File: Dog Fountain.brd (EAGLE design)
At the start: 88.6 x 53.3 mm, 19 parts, among them IC1 L298, J1 22-27-2021-02, J4 22-27-2021-02

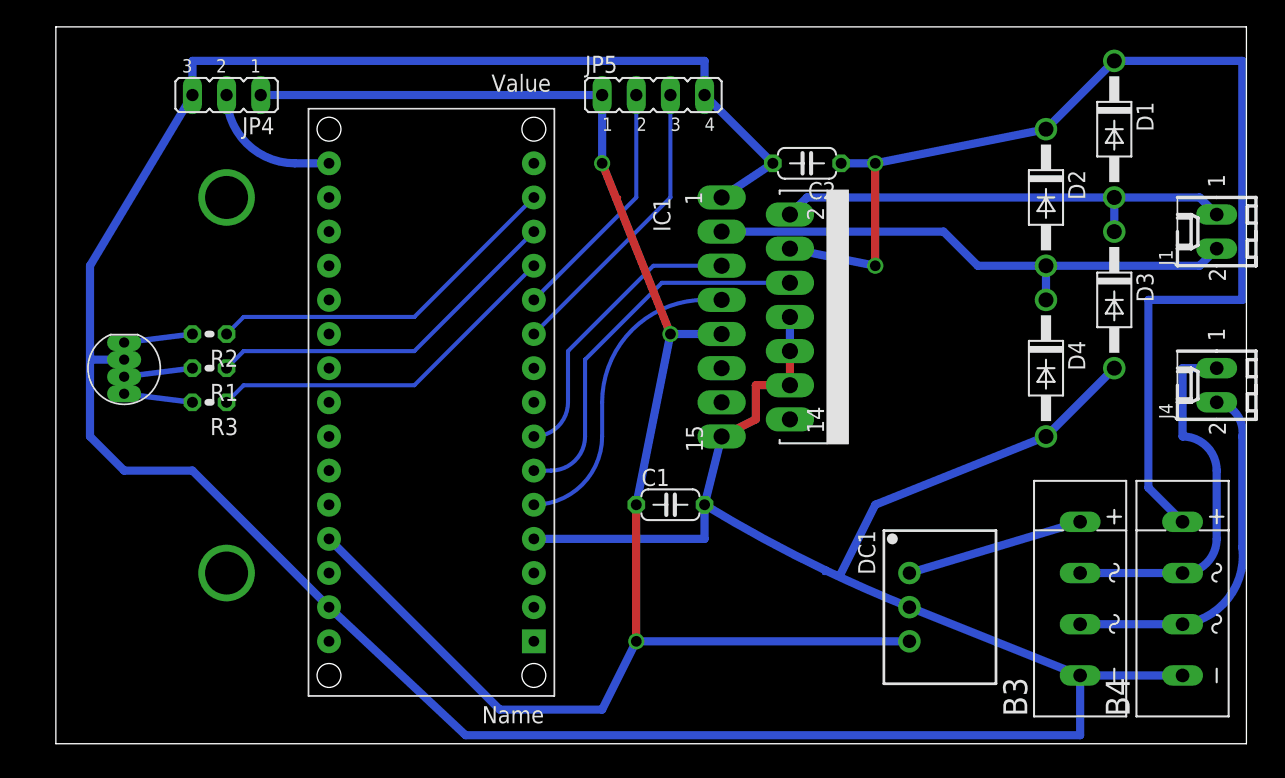
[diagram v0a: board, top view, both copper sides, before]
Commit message: PCB board first test
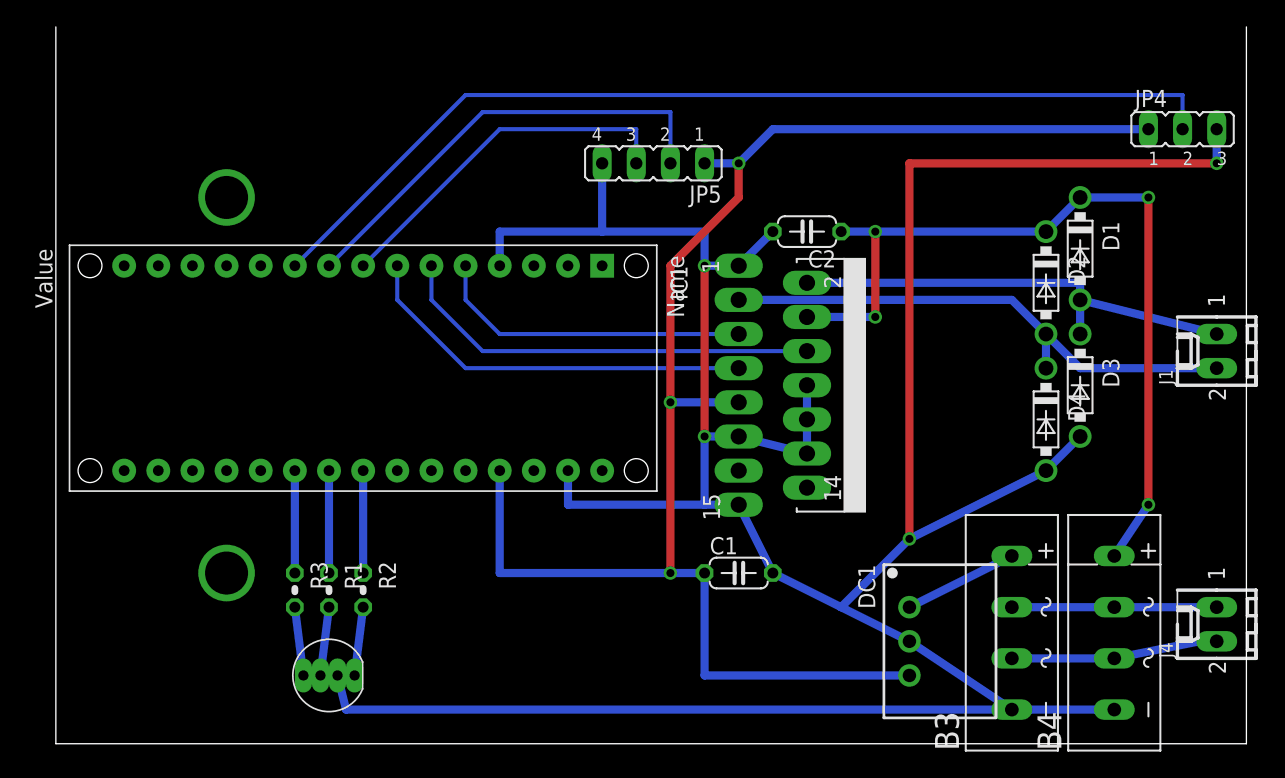
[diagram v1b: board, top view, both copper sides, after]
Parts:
- D1, D2, D3, D4: device diode:DO41-10 -> diode:DO41-7.6
- R1, R3: value (none) -> 100 Ω
- R2: value (none) -> 180 Ω
- moved JP4 71.2 mm to (83.8, 45.7), turned to 0 degrees
- moved U$1 31.4 mm to (43.2, 35.6), turned to 270 degrees
- moved D5 27.5 mm to (20.3, 5.08), turned to 0 degrees
- moved R2 22.2 mm to (22.9, 11.4), turned to 270 degrees
- moved R1 18.8 mm to (20.3, 11.4), turned to 270 degrees
- moved J4 17.8 mm to (86.4, 8.89)
- moved R3 15.3 mm to (17.8, 11.4), turned to 270 degrees
- moved D1 9.25 mm to (76.2, 36.8)
- moved J1 8.89 mm to (86.4, 29.2)
- moved C1 7.18 mm to (50.8, 12.7)
- moved D3 6.84 mm to (76.2, 26.7)
- moved D2 6.35 mm to (73.7, 34.3)
- moved B3 5.68 mm to (71.1, 8.26)
- moved B4 5.68 mm to (78.7, 8.26)
- moved IC1 5.24 mm to (58.4, 26.7)
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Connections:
- net N$11: now also U$1.D7; no longer U$1.D13
- net N$12: now also U$1.D6; no longer U$1.D8
- net N$13: now also U$1.D5; no longer U$1.D7
- net N$14: now also U$1.A5; no longer U$1.D9
- net N$15: now also U$1.A4; no longer U$1.D10
- net N$16: now also U$1.A3; no longer U$1.D11
- net N$5: now also U$1.D2; no longer U$1.D4
- net N$8: now also U$1.D4; no longer U$1.D2
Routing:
- net N$11: track 9.72 -> 73.8 mm
- net GND: track 272.0 -> 238.8 mm, vias 0 -> 4
- net +24V: track 88.6 -> 62.8 mm, vias 0 -> 3
- net N$15: track 27.1 -> 7.62 mm
- net N$14: track 27.1 -> 7.62 mm
- net N$16: track 27.1 -> 7.62 mm
- net N$12: track 18.4 -> 33.9 mm
- net N$10: track 27.5 -> 15.2 mm
- net N$9: track 26.3 -> 15.4 mm
- net N$8: track 21.8 -> 30.0 mm
- net +5V: track 122.9 -> 117.5 mm, vias 2 -> 3
- net N$13: track 22.0 -> 27.1 mm
- net N$3: track 13.3 -> 8.52 mm
- net N$4: track 28.2 -> 32.1 mm
- net N$5: track 21.5 -> 23.9 mm
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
